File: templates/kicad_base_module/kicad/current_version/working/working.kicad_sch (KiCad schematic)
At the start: 2 parts, among them U1 itq32at328

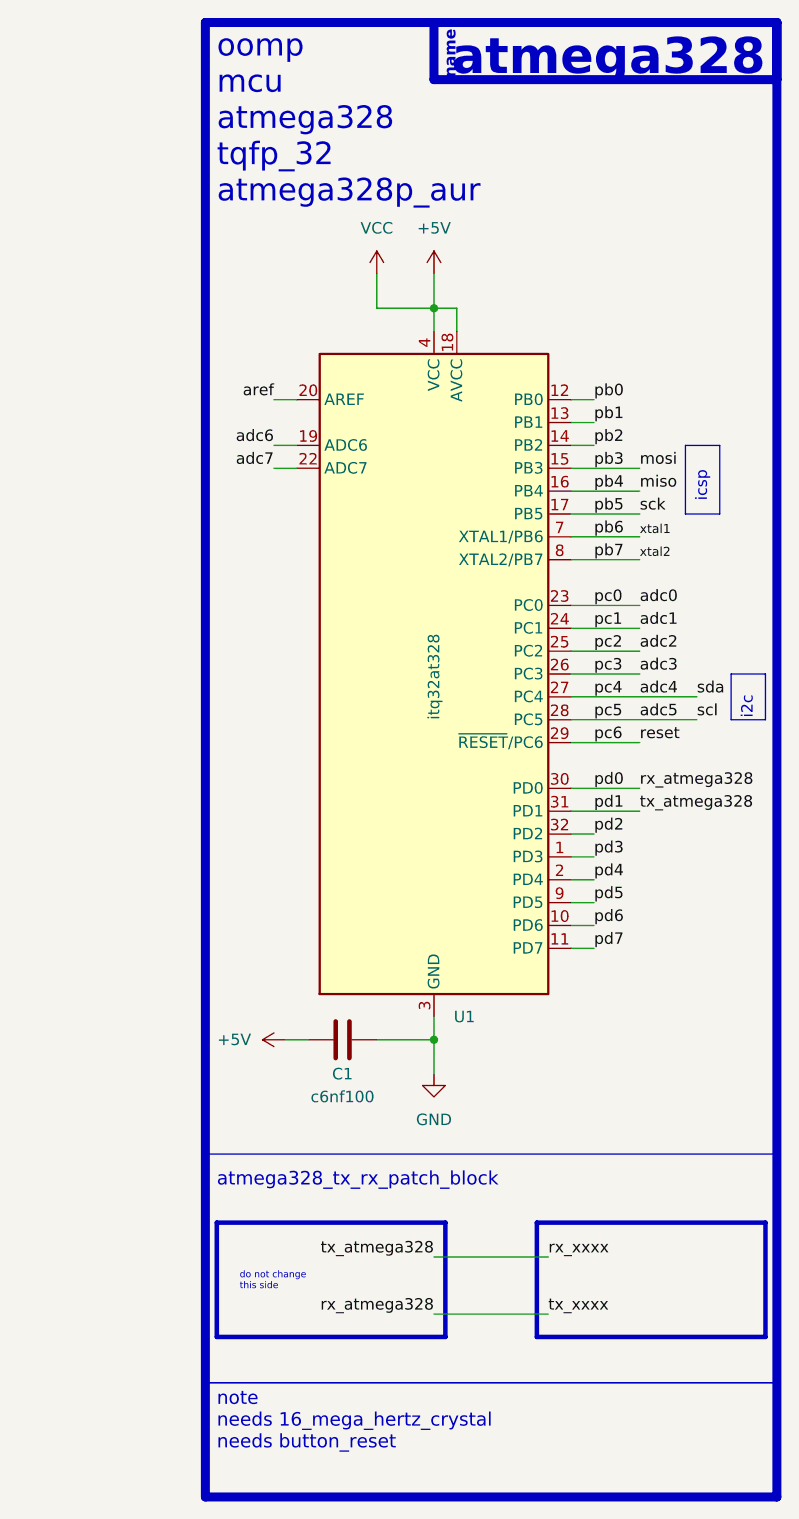
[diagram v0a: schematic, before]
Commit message: template work
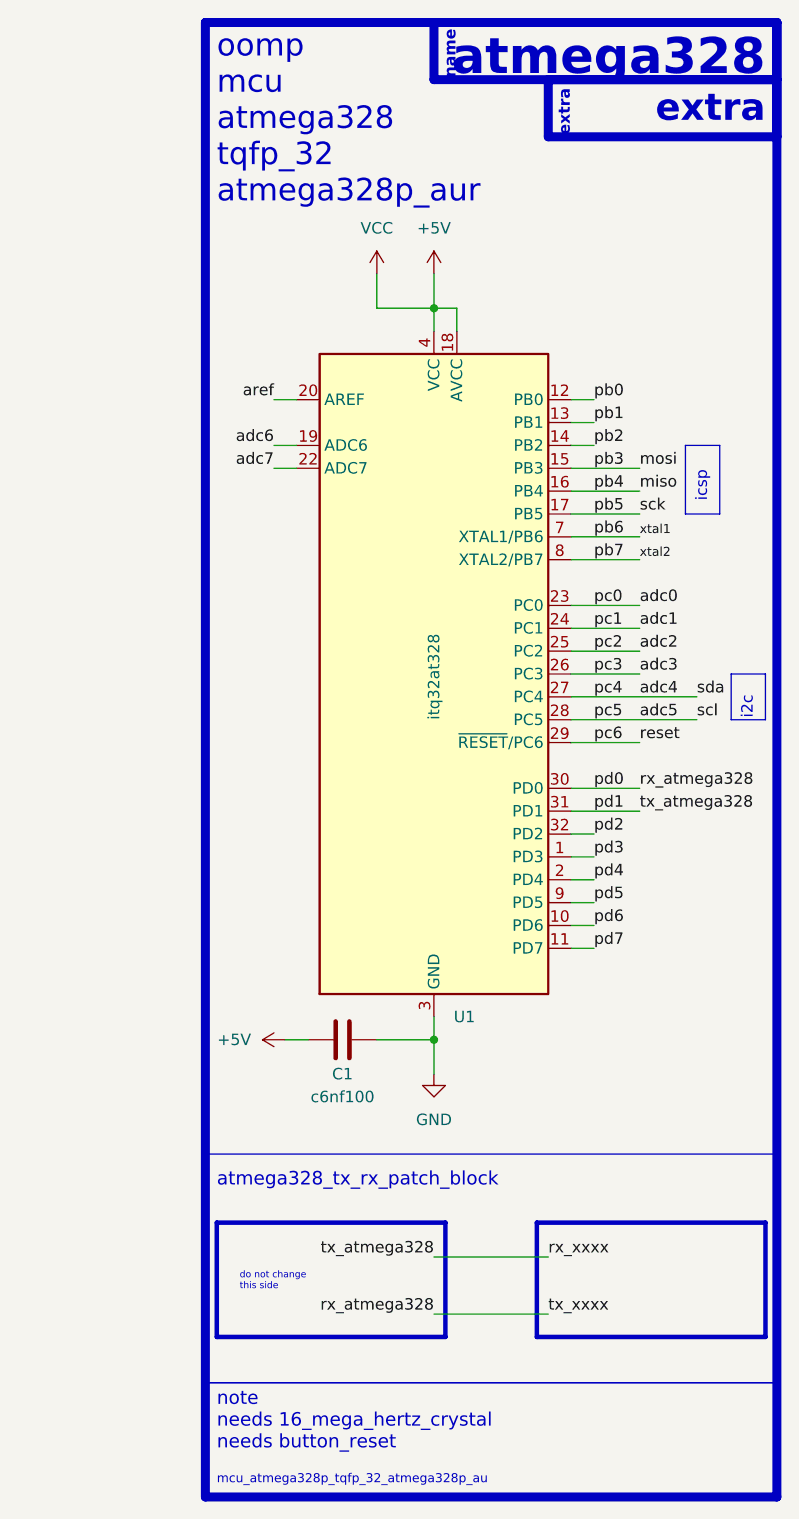
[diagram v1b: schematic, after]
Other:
- note added: "extra"
- note added: "mcu_atmega328p_tqfp_32_atmega328p_au"
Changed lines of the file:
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@@
+    (fill (type none))
+  )
+  (rectangle (start 132.08 24.13) (end 157.48 30.48)
+    (stroke (width 1) (type default))
     (fill (type none))
   )
@@
     (effects (font (size 1.27 1.27)) (justify left bottom))
   )
+  (text "mcu_atmega328p_tqfp_32_atmega328p_au" (at 95.25 180.34 0)
+    (effects (font (size 1 1)) (justify left bottom))
+  )
   (text "atmega328" (at 156.21 24.13 0)
     (effects (font (size 4 4) (thickness 0.8) bold (color 255 255 255 1)) (justify right bottom))
@@
     (effects (font (size 1.5 1.5)) (justify left bottom))
   )
+  (text "extra" (at 156.21 29.21 0)
+    (effects (font (size 3 3) (thickness 0.8) bold) (justify right bottom))
+  )
   (text "oomp\nmcu\natmega328\ntqfp_32\natmega328p_aur" (at 95.25 38.1 0)
     (effects (font (size 2.5 2.5)) (justify left bottom))
   )
+  (text "extra" (at 134.62 30.48 90)
+    (effects (font (size 1.27 1.27) (thickness 0.254) bold) (justify left bottom))
+  )
   (text "atmega328_tx_rx_patch_block" (at 95.25 147.32 0)

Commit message: fixed up template and others
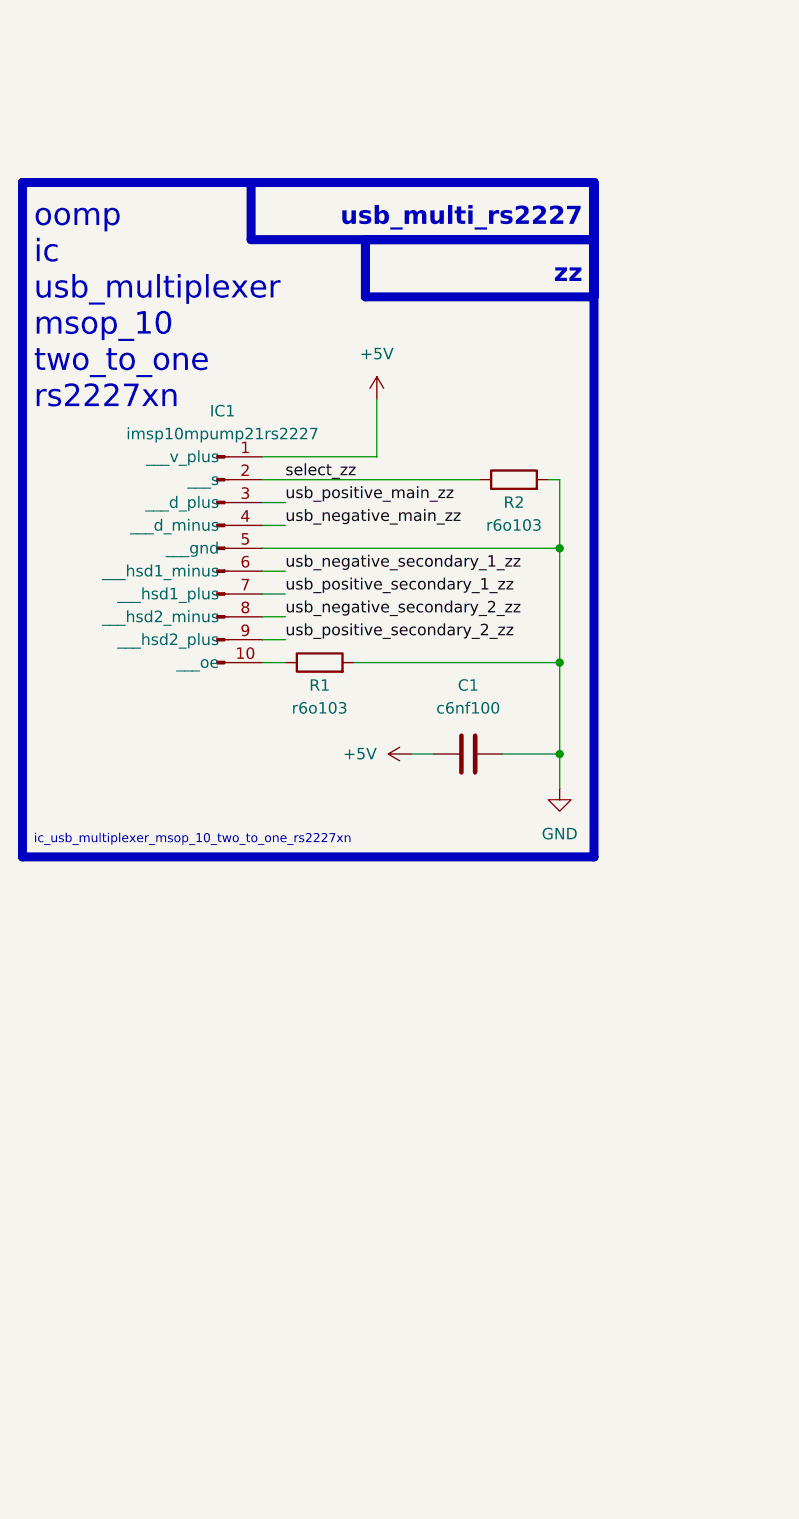
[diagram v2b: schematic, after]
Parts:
- removed U1: itq32at328, oomlout_oomp_part_kicad_footprints:itq32at328_electronic_ic_tqfp_32_mcu_atmega328_microchip_atmega328p_aur, symbol oomlout_oomp_part_symbols:itq32at328_electronic_ic_tqfp_32_mcu_atmega328_microc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
- added IC1: imsp10mpump21rs2227, oomlout_oomp_part_footprints:imsp10mpump21rs2227_electronic_ic_msop_10_multiplexer_usb_multiplexer_two_to_one_jiangsu_r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, symbol oomlout_oomp_part_symbols:imsp10mpump21rs2227_electronic_ic_msop_10_multiplexer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
- added R1, R2: r6o103, oomlout_oomp_part_footprints:r6o103_electronic_resistor_0603_10000_ohm, symbol oomlout_oomp_part_symbols:r6o103_electronic_resistor_0603_10000_ohm
- C1: footprint oomlout_oomp_part_kicad_footprints:c6nf100_electronic_capacitor_0603_100_nano_farad -> oomlout_oomp_part_footprints:c6nf100_electronic_capacitor_0603_100_nano_farad
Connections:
- net +5V: now also IC1.1 (___v_plus)
- net GND: now also IC1.5 (___gnd), R1.2, R2.2
- new net: IC1.10 (___oe), R1.1
- new net select_zz: IC1.2 (___s), R2.1
- new net usb_negative_main_zz: IC1.4 (___d_minus)
- new net usb_negative_secondary_1_zz: IC1.6 (___hsd1_minus)
- new net usb_negative_secondary_2_zz: IC1.8 (___hsd2_minus)
- new net usb_positive_main_zz: IC1.3 (___d_plus)
- new net usb_positive_secondary_1_zz: IC1.7 (___hsd1_plus)
- new net usb_positive_secondary_2_zz: IC1.9 (___hsd2_plus)
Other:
- note added: "ic_usb_multiplexer_msop_10_two_to_one_rs2227xn"
- note added: "oomp ic usb_multiplexer msop_10 two_to_one rs2227xn"
- note added: "usb_multi_rs2227"
- note added: "zz"
- note removed: "atmega328"
- note removed: "atmega328_tx_rx_patch_block"
- note removed: "do not change this side"
- note removed: "extra"
- note removed: "i2c"
- note removed: "icsp"
- note removed: "mcu_atmega328p_tqfp_32_atmega328p_au"
- note removed: "name"
- note removed: "note needs 16_mega_hertz_crystal needs button_reset"
- note removed: "oomp mcu atmega328 tqfp_32 atmega328p_aur"
